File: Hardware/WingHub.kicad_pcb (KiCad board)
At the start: 2 copper layers, 50.8 x 22.9 mm, 19 parts, among them J1 feather long, J2 feather short, J3 USB_A, SW2 DOWNLOADER, U1 CH559T

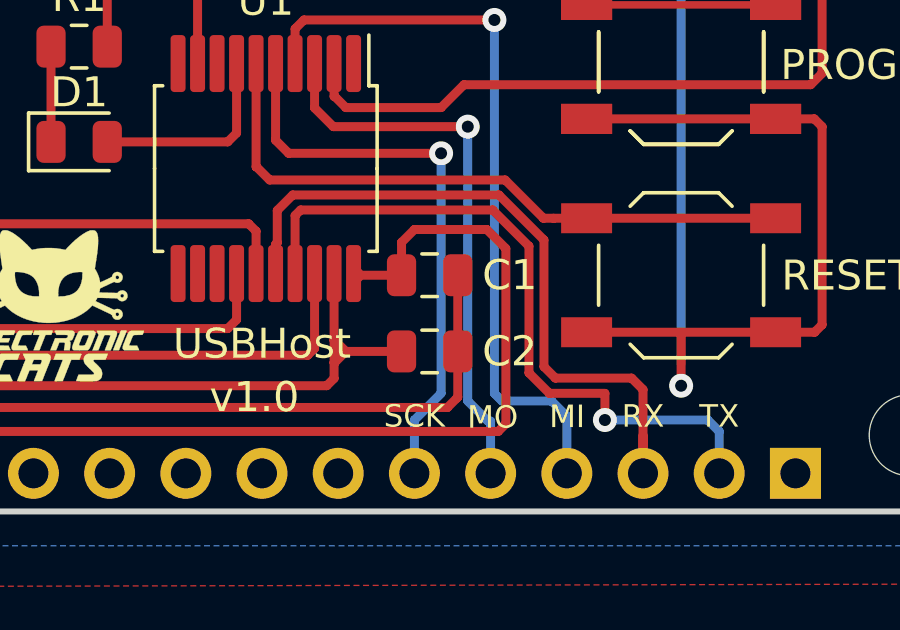
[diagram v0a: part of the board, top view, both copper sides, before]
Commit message: WingHubBom.ods created with plugin.
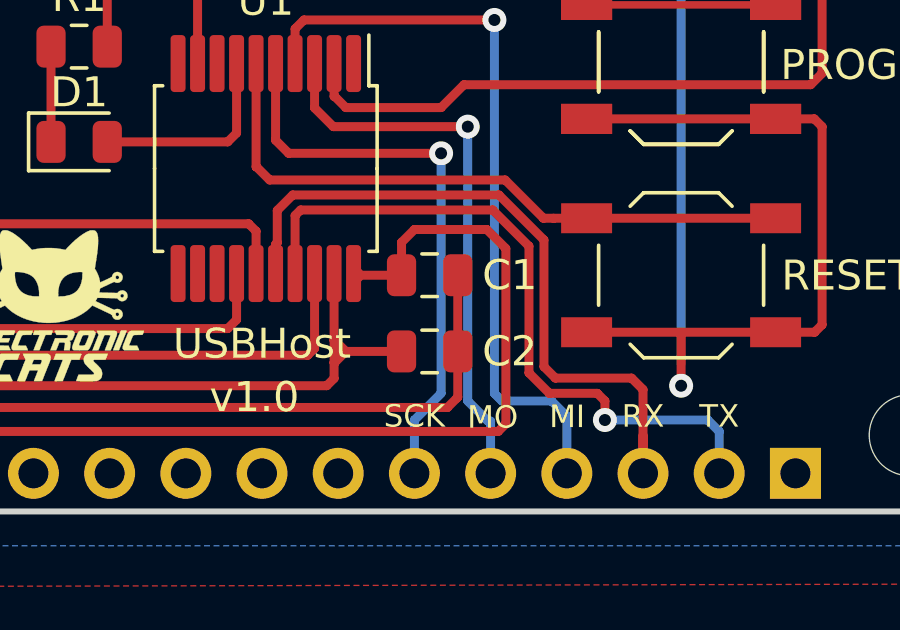
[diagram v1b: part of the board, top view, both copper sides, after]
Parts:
- removed the J3 at (39.1, 33.3) (x2)
- added J3 (x2): USB_A, Connector_USB:USB_A_CONNFLY_DS1095-WNR0, F.Cu at (39.1, 33.3)

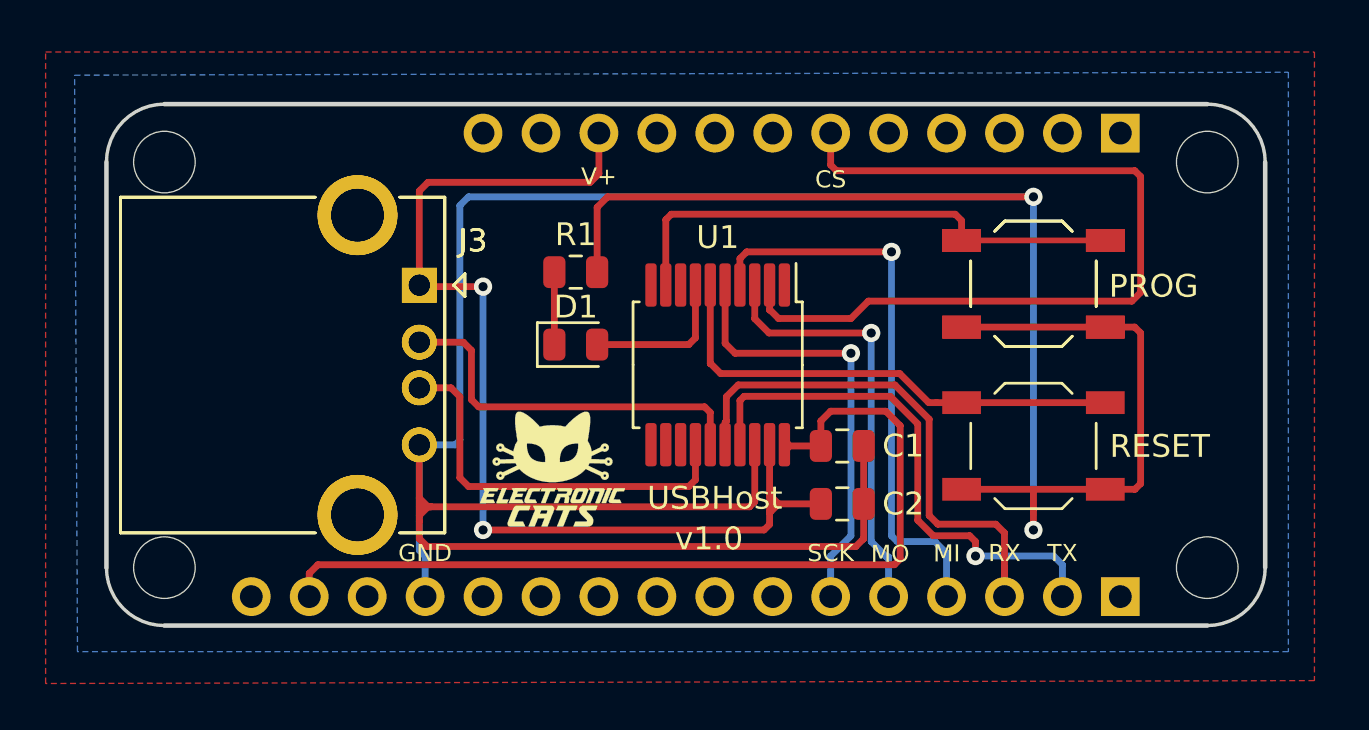
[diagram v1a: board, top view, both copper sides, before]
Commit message: Hardware changes added
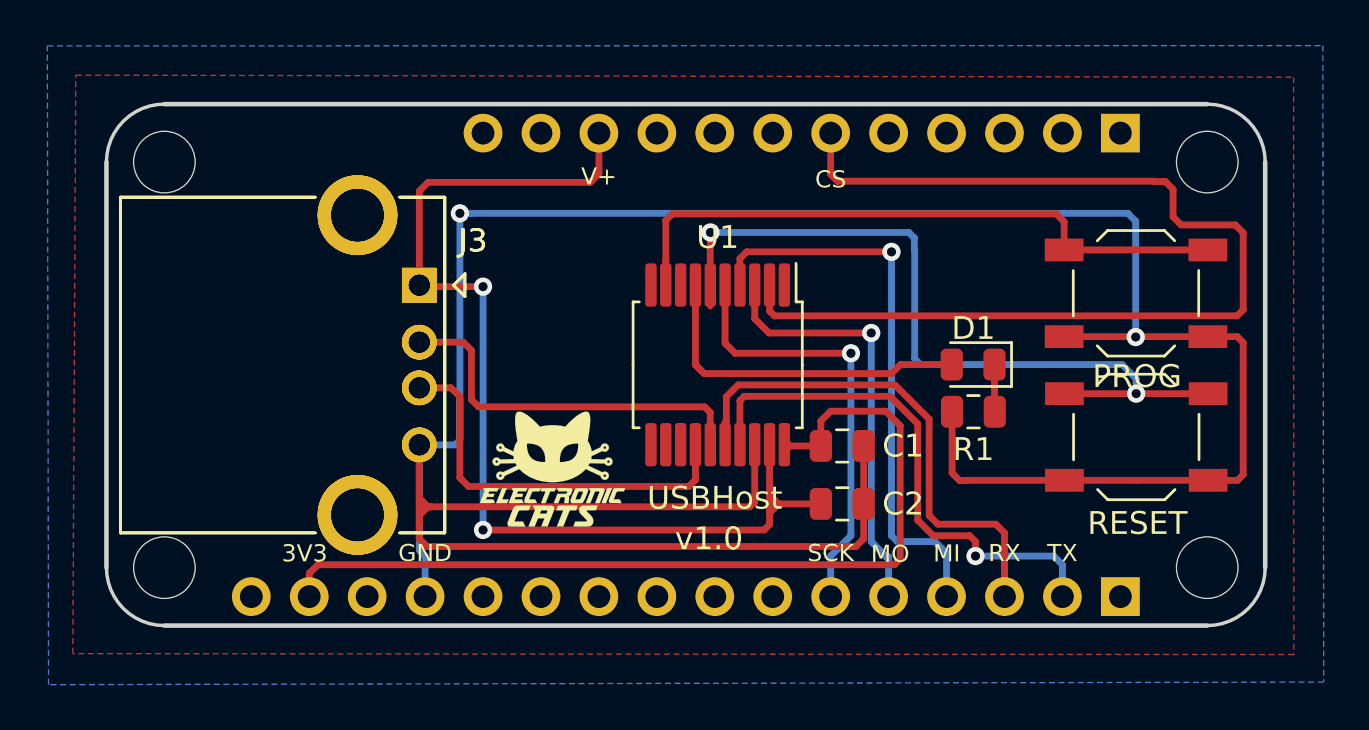
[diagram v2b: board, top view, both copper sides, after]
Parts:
- removed the J3 at (39.1, 33.3) (x2)
- removed SW2: DOWNLOADER, Button_Switch_SMD:SW_SPST_TL3342
- added J3 (x2): USB_A, Connector_USB:USB_A_CONNFLY_DS1095-WNR0, F.Cu at (39.1, 33.3)
- moved R1 18.5 mm to (63.4, 38.9), turned to 180 degrees
- moved D1 17.4 mm to (63.4, 36.8), turned to 180 degrees
- moved RESET 4.53 mm to (70.5, 40.0)
- moved PROG 4.52 mm to (70.5, 33.7)
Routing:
- net GND: track 152.6 -> 130.3 mm
- net /RST: track 22.4 -> 34.6 mm, vias 0 -> 2
- net /CS: track 38.3 -> 47.1 mm
- net /LED: track 6.75 -> 15.2 mm
- net /PROG: track 24.3 -> 29.2 mm
- net Net-(D1-Pad1): track 3.18 -> 2.08 mm
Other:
- board text added: "3V3"
